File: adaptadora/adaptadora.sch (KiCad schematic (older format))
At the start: 39 parts, among them J1 Conn_Coaxial, J10 Conn_01x02, J11 Conn_Coaxial, J12 Conn_Coaxial, J2 Conn_Coaxial, J3 Conn_Coaxial, J4 Conn_Coaxial, J5 Conn_Coaxial, J6 Conn_01x02, J7 Conn_02x20_Odd_Even, J8 Conn_02x20_Odd_Even, J9 Conn_01x04, U1 LM361MX_NOPB-LM361MX_NOPB, U2 TLV2772IDR

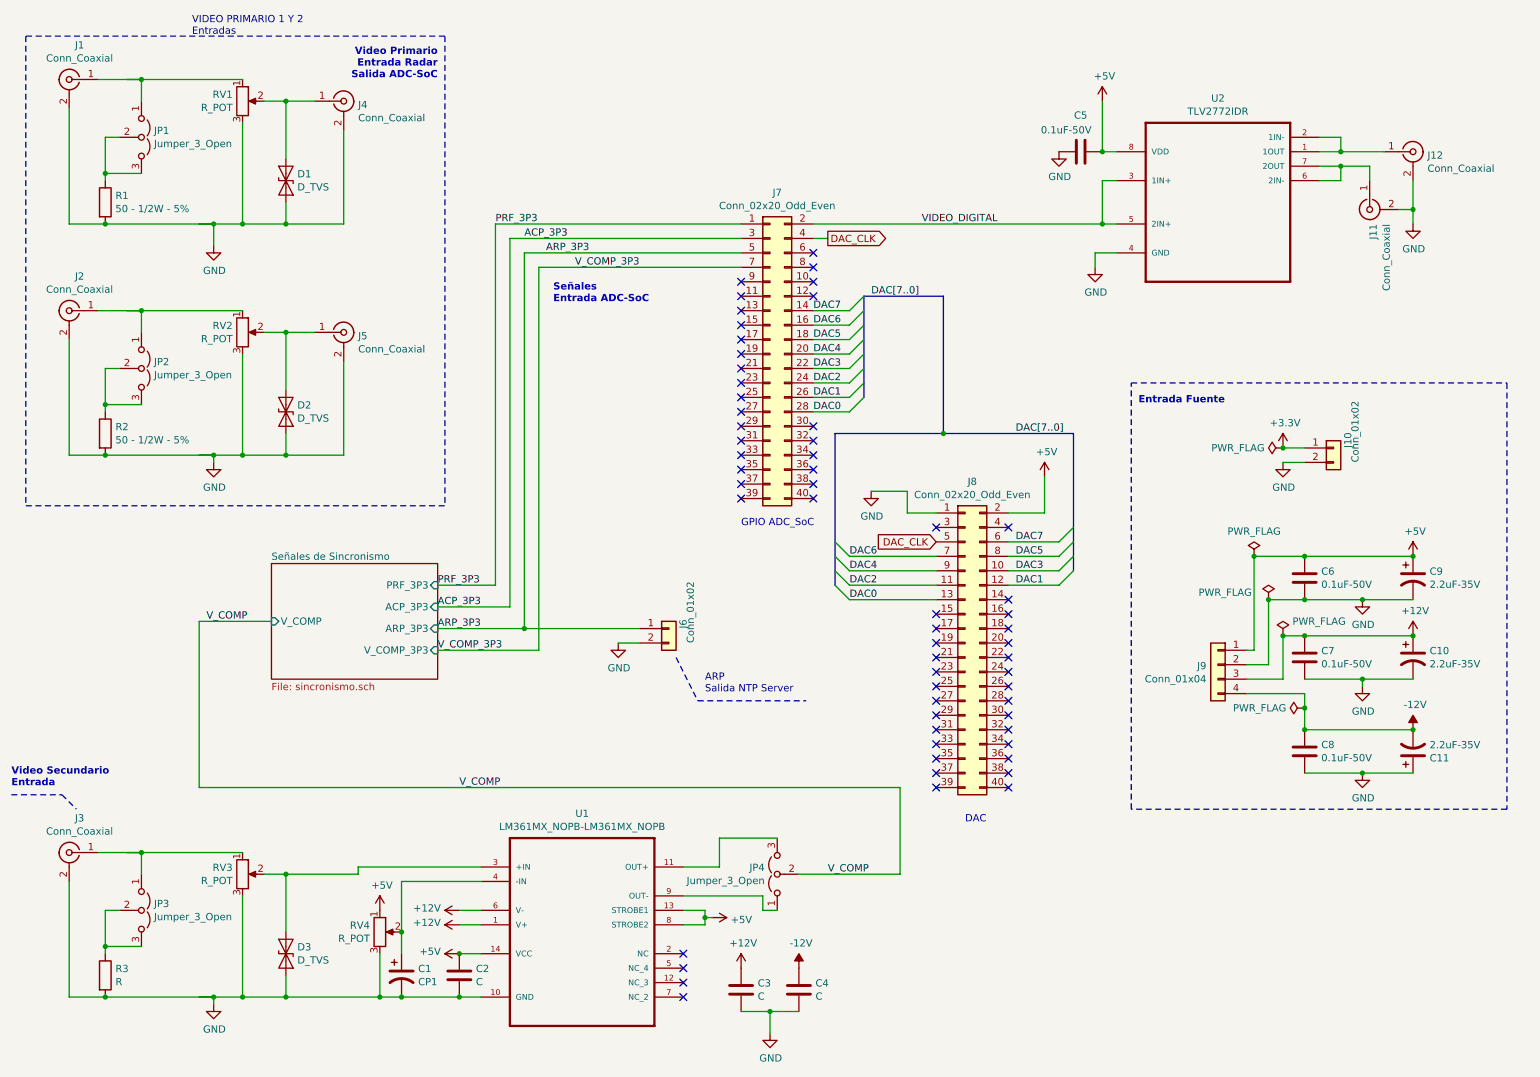
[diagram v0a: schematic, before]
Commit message: work in progress
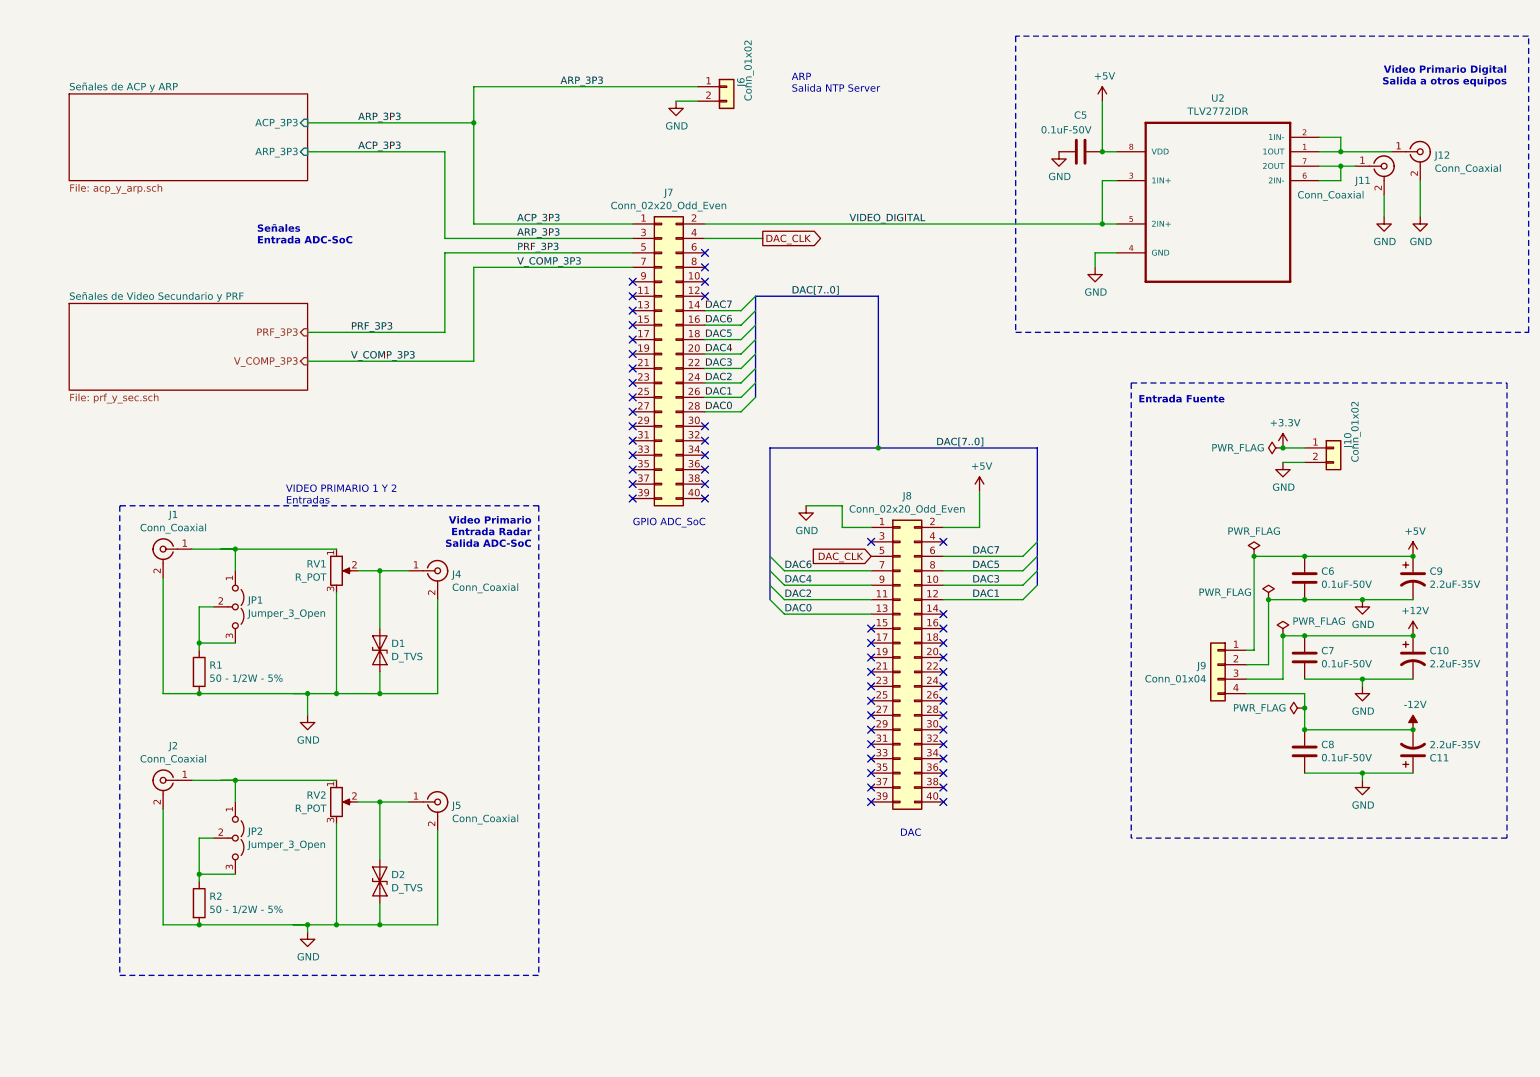
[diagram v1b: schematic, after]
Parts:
- removed C1: CP1, symbol Device:CP1
- removed C2, C3, C4: C, symbol Device:C
- removed D3: D_TVS, symbol Device:D_TVS
- removed J3: Conn_Coaxial, symbol Connector:Conn_Coaxial
- removed JP3, JP4: Jumper_3_Open, symbol Jumper:Jumper_3_Open
- removed R3: R, symbol Device:R
- removed RV3, RV4: R_POT, symbol Device:R_POT
- removed U1: LM361MX_NOPB-LM361MX_NOPB, SOIC127P600X175-14N, symbol sincronismo-rescue:LM361MX_NOPB-LM361MX_NOPB
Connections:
- net labels removed: V_COMP
- wire segments 176 -> 124
- no-connect marks 59 -> 55
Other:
- note added: "Video Primario Digital\nSalida a otros equipos"
- note removed: "Video Secundario\nEntrada"
- moved on the sheet: D1, D2, J1, J11, J12, J2, J4, J5, J6, J7, J8, JP1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
